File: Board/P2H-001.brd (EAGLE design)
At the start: 72 x 72 mm, 27 parts, among them IC1 74LS157N, IC2 LTC485N, IC3 4051N, IC4 74LS07N, IC5 LTC485N, U1 ARDUINO_PRO_MINI, U2 MAX7219DIP

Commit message: Refinement of panel and schematic.
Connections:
- net SEL0: no longer U1.A6
- net SEL1: now also U1.A6
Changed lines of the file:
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@@
 </signal>
 <signal name="SEL0">
-<contactref element="U1" pad="A6"/>
 <contactref element="IC3" pad="11"/>
 <wire x1="64.6938" y1="59.6646" x2="58.5216" y2="65.8368" width="0.254" layer="1"/>
@@
 <wire x1="42.291" y1="37.9476" x2="48.2346" y2="37.9476" width="0.254" layer="16"/>
 <wire x1="58.5216" y1="65.8368" x2="58.42" y2="66.04" width="0.254" layer="1"/>
-<wire x1="42.291" y1="37.9476" x2="42.06875" y2="37.7825" width="0.254" layer="16"/>
 <via x="51.6636" y="41.3766" extent="1-16" drill="0.6096"/>
 </signal>
 <signal name="SEL1">
-<contactref element="U1" pad="A7"/>
 <contactref element="IC3" pad="10"/>
 <wire x1="60.8076" y1="63.0936" x2="60.8076" y2="65.8368" width="0.254" layer="16"/>
@@
 <wire x1="39.5478" y1="37.9476" x2="40.6908" y2="39.0906" width="0.254" layer="16"/>
 <wire x1="60.8076" y1="65.8368" x2="60.96" y2="66.04" width="0.254" layer="16"/>
-<wire x1="39.5478" y1="37.9476" x2="39.52875" y2="37.7825" width="0.254" layer="16"/>
 <via x="57.3786" y="53.4924" extent="1-16" drill="0.6096"/>
 <via x="58.293" y="50.292" extent="1-16" drill="0.6096"/>
+<contactref element="U1" pad="A6"/>
+<contactref element="U1" pad="A7"/>
+<wire x1="40.6908" y1="39.0906" x2="42.06875" y2="37.7825" width="0" layer="19" extent="16-16"/>
+<wire x1="39.52875" y1="37.7825" x2="39.5478" y2="37.9476" width="0" layer="19" extent="16-16"/>
 </signal>
 <signal name="I2C0">

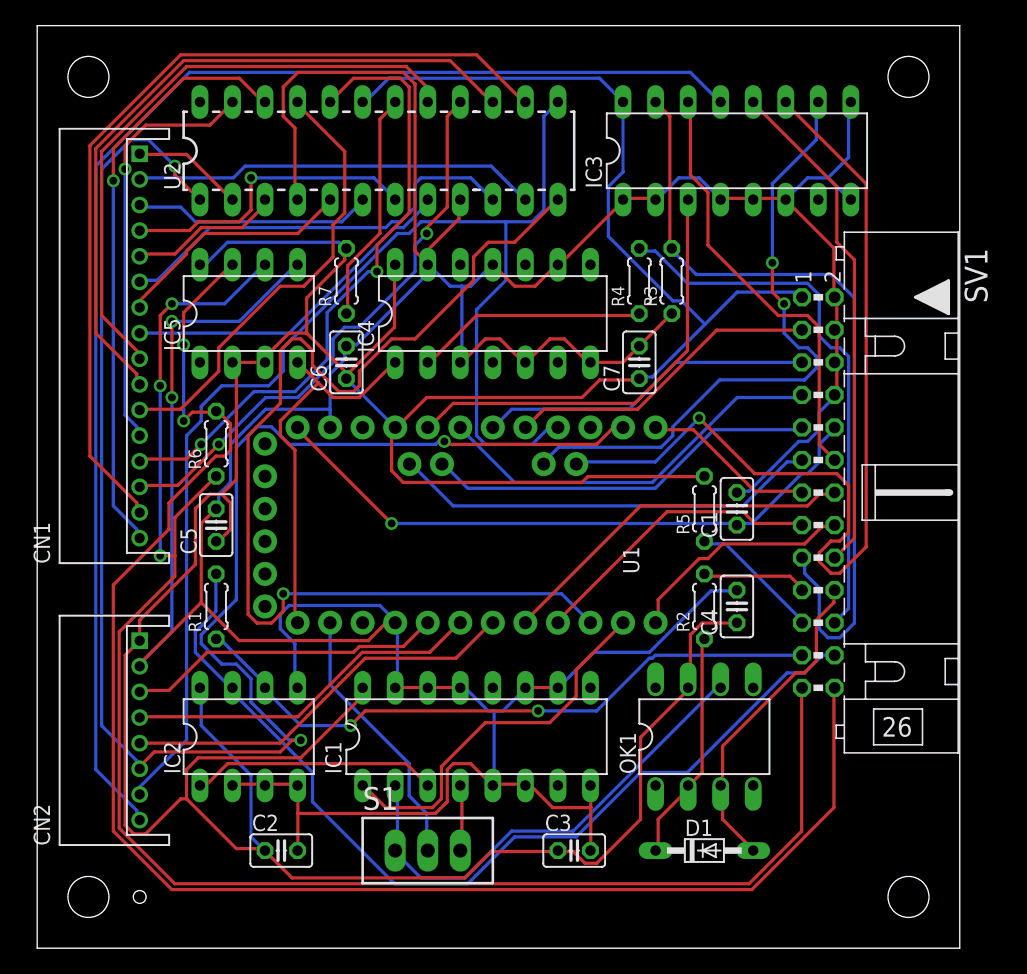
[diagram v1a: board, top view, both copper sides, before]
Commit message: Before the first prototyping.
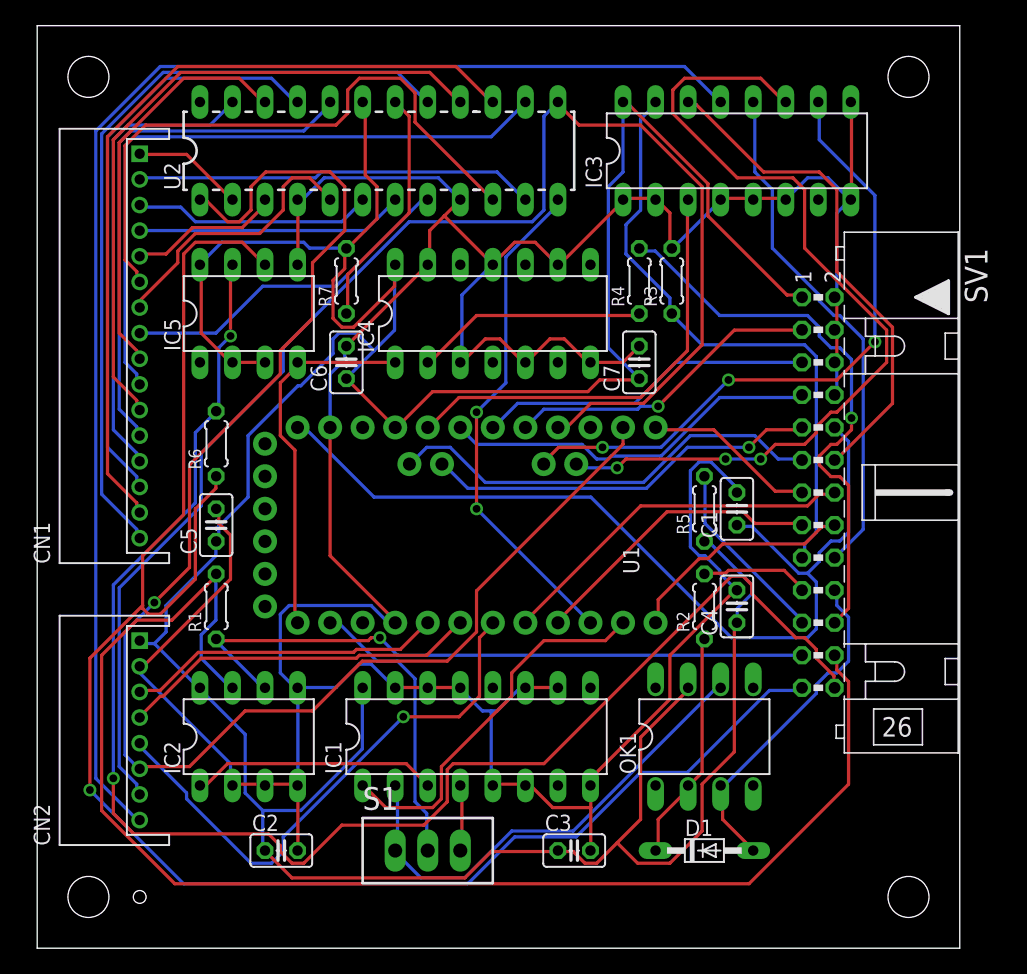
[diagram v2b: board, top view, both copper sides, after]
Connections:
- net DIG0 renamed LIGHTPORT1
- net DIG1 renamed LIGHTPORT2
- net DIG2 renamed LIGHTPORT3
- net DIG3 renamed LIGHTPORT4
- net DIG4 renamed LIGHTPORT5
- net DIG5 renamed LIGHTPORT6
- net DIG6 renamed LIGHTPORT7
- net DIG7 renamed LIGHTPORT8
- net GDETECT renamed DETECT1
- net M0 renamed MIDI4
- net M1 renamed MIDI5
- net M2 renamed MIDI6
- net M3 renamed MIDI7
- net RXA renamed MIDI0
- net RXK renamed MIDI1
- net SWMAIN renamed S3
- net SWMAX renamed S4
- net SWMIN renamed S5
- net TXSNK renamed MIDI3
- net VDETECT renamed DETECT0
- net XDETECT renamed DETECT3
- removed net MDETECT: IC3.15, R3.2, SV1.17
- removed net N$3: R5.1, SV1.21
- removed net SEG0: CN1.9, U2.17
- removed net SEG1: CN1.10, U2.15
- removed net SEG2: CN1.11, U2.21
- removed net SEG3: CN1.12, U2.23
- removed net SEG4: CN1.13, U2.20
- removed net SEG5: CN1.14, U2.16
- removed net SEG6: CN1.15, U2.14
- removed net SEG7: CN1.16, U2.22
- removed net SEL0: IC3.11
- removed net SEL1: IC3.10, U1.A6, U1.A7
- new net DETECT2: IC3.15, R3.1, SV1.17
- new net LIGHTPORT10: CN1.10, U2.14
- new net LIGHTPORT11: CN1.11, U2.16
- new net LIGHTPORT12: CN1.12, U2.20
- new net LIGHTPORT13: CN1.13, U2.23
- new net LIGHTPORT14: CN1.14, U2.21
- new net LIGHTPORT15: CN1.15, U2.15
- new net LIGHTPORT16: CN1.16, U2.17
- new net LIGHTPORT9: CN1.9, U2.22
- new net MIDI2: R5.2, SV1.21
- new net SELECT0: IC3.11, U1.A6
- new net SELECT1: IC3.10, U1.A7
- net GND: now also R3.2; no longer R3.1
- net VCC: now also R5.1; no longer R5.2
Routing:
- net SEL0: track 74.1 -> 0.00 mm, vias 1 -> 0
- net SEG6: track 68.8 -> 0.00 mm
- net SELECT0: track 0.00 -> 68.7 mm, vias 0 -> 3
- net LIGHTPORT15: track 0.00 -> 63.9 mm
- net MDETECT: track 63.0 -> 0.00 mm
- net LIGHTPORT16: track 0.00 -> 61.3 mm
- net GND: track 349.8 -> 294.4 mm, vias 2 -> 0
- net SEG1: track 55.0 -> 0.00 mm
- net LIGHTPORT11: track 0.00 -> 52.2 mm
- net LIGHTPORT10: track 0.00 -> 51.8 mm
- net SELECT1: track 0.00 -> 50.4 mm, vias 0 -> 3
- net SEG4: track 49.6 -> 0.00 mm, vias 2 -> 0
- net SEL1: track 48.8 -> 0.00 mm, vias 2 -> 0
- net DETECT2: track 0.00 -> 47.8 mm
- net SEG0: track 47.4 -> 0.00 mm
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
